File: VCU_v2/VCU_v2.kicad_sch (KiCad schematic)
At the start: 0 parts

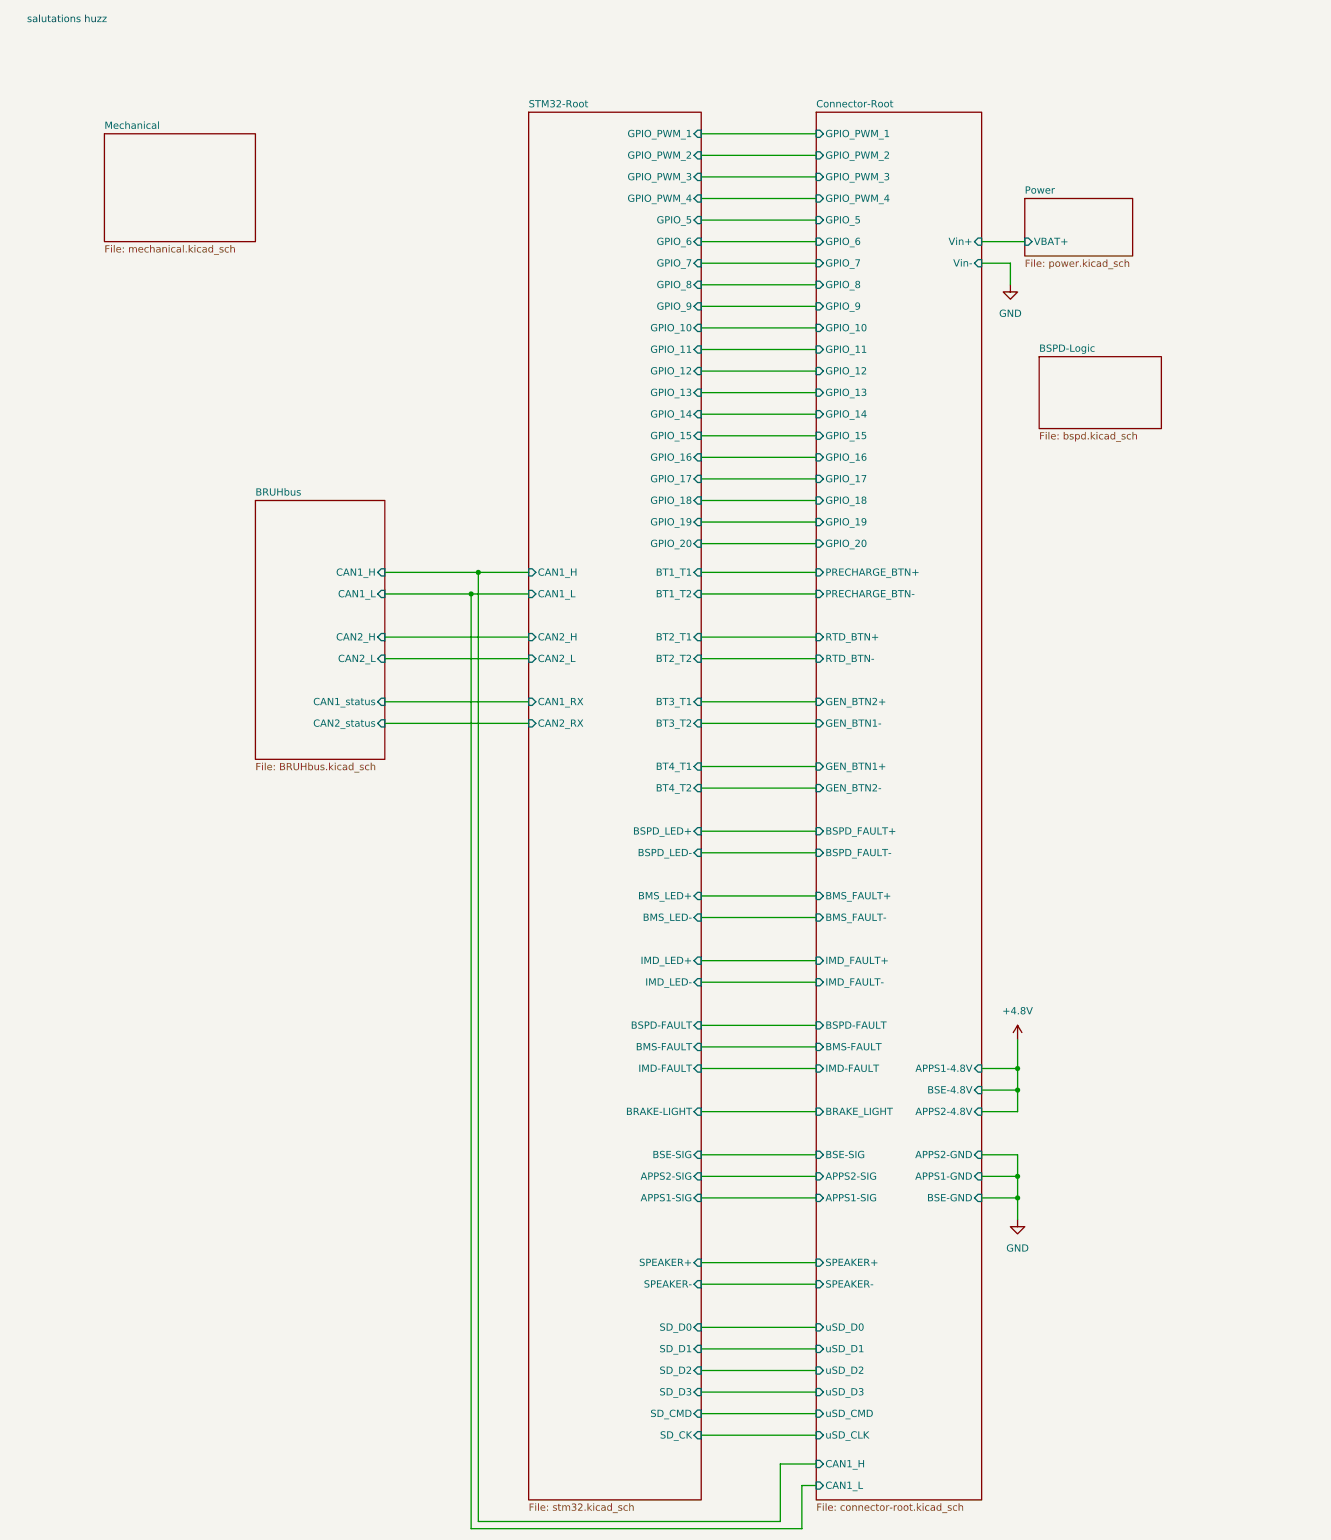
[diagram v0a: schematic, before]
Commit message: bspd schematic done
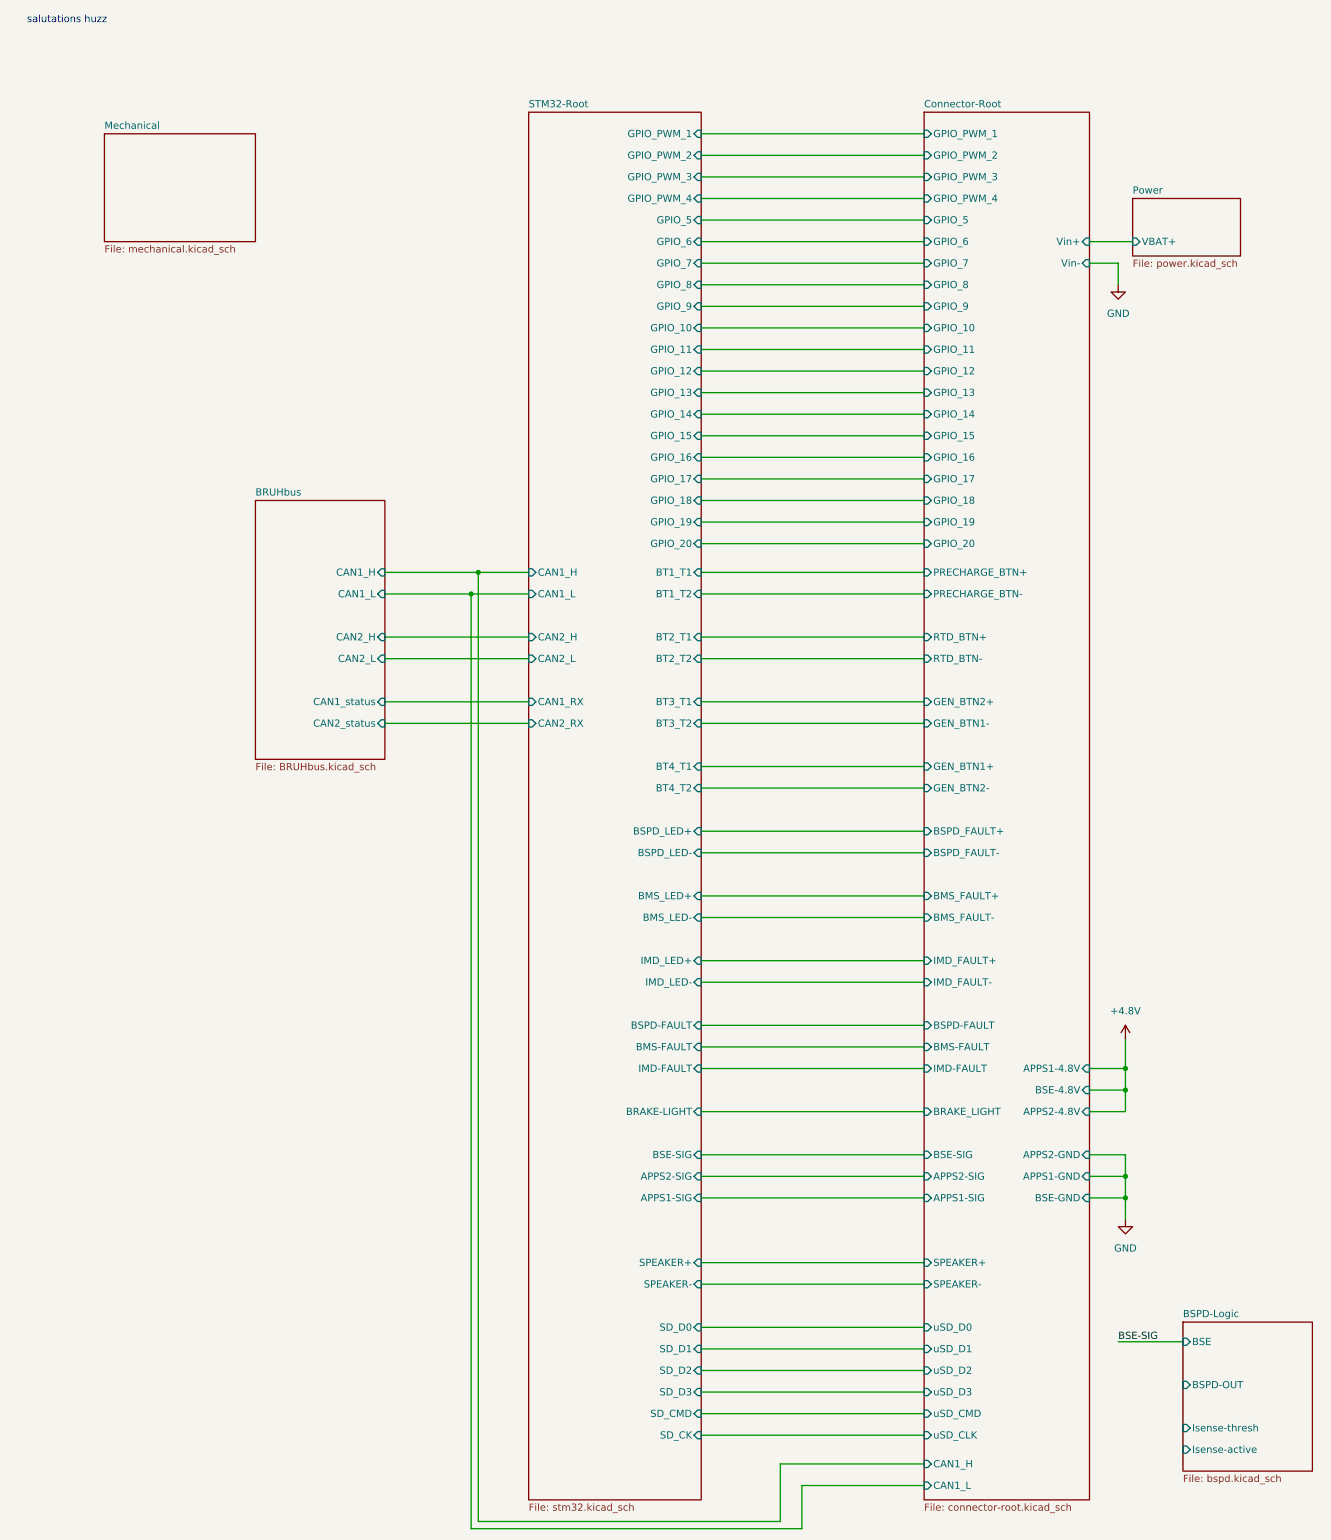
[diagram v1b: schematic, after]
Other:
- sheet BSPD-Logic ports: added BSE, BSPD-OUT, Isense-active, Isense-thresh; removed none
